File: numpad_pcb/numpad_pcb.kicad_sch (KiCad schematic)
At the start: 35 parts, among them J1 numpad, J10 Conn_01x02, J11 Conn_01x02, J12 Conn_01x02, J13 Conn_01x02, J14 Conn_01x02, J15 Conn_01x02, J17 Conn_01x02, J2 Conn_01x02, J3 Conn_01x02, J4 Conn_01x02, J6 Conn_01x02, J7 Conn_01x02, J8 Conn_01x02, J9 Conn_01x02, U1 ProMicro

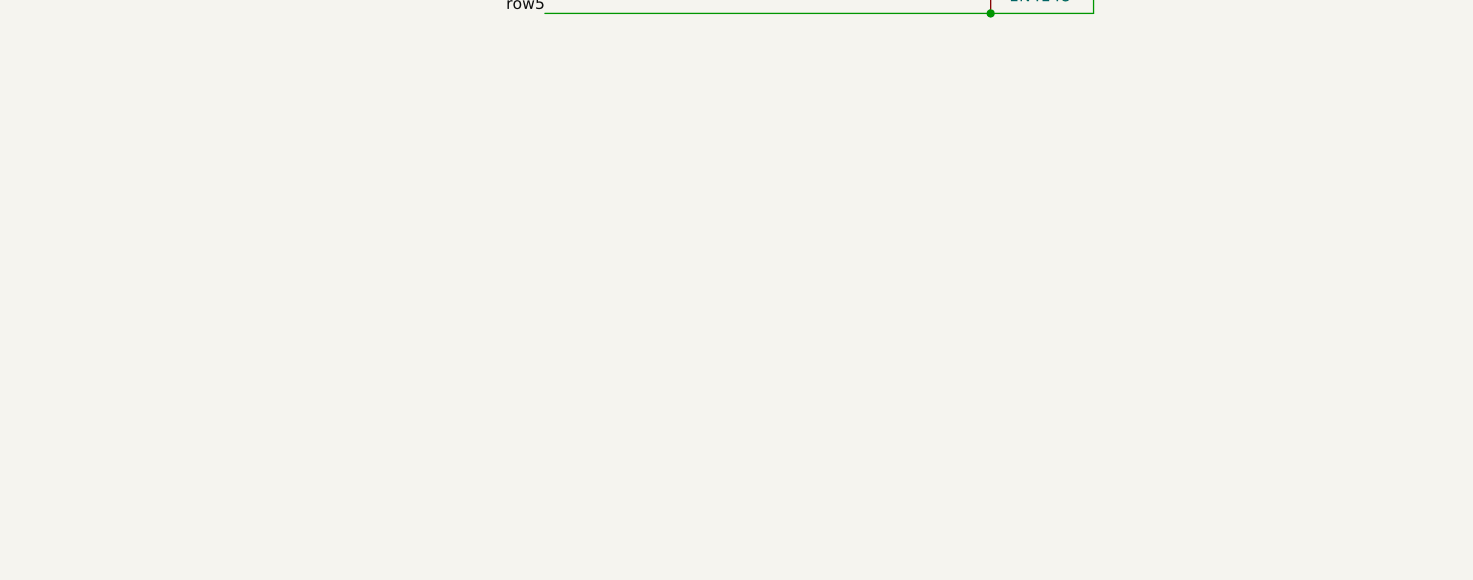
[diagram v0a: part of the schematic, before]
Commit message: tweaked silk, added todo for upgraded layout, added config
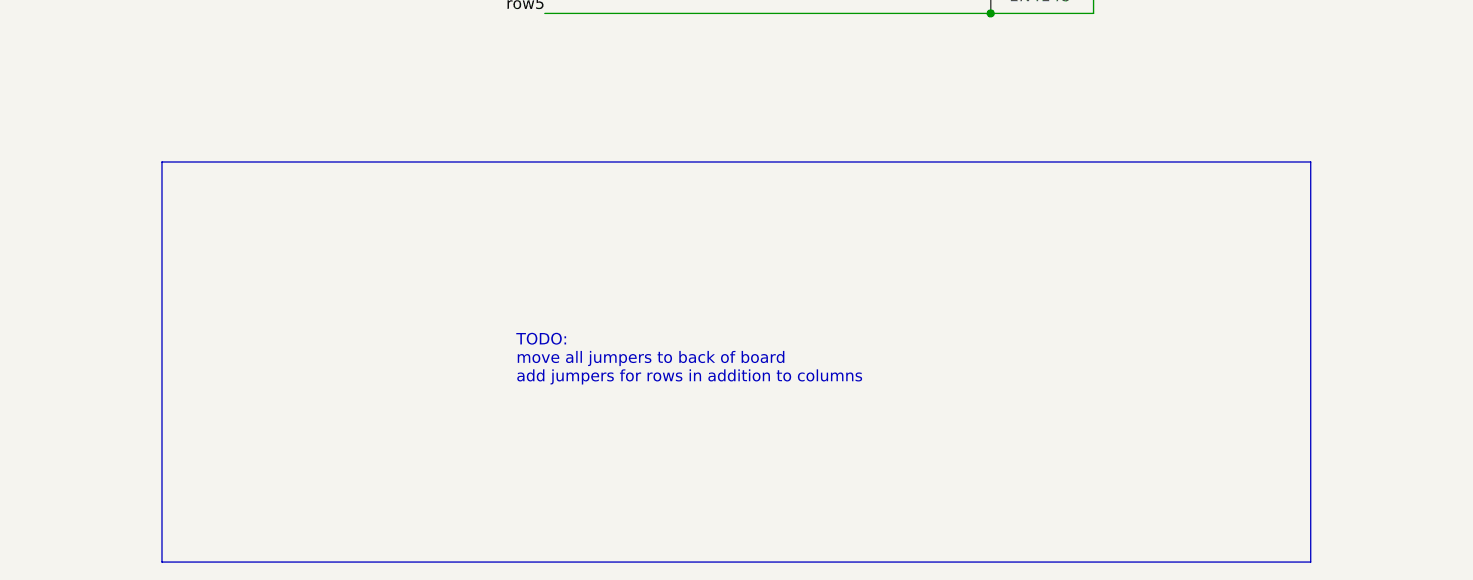
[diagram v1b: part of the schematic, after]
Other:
- note added: "TODO: move all jumpers to back of board add jumpers for rows in addition to columns"
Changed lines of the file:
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@@
+    (stroke (width 0) (type default) (color 0 0 0 0))
+  )
+  (polyline (pts (xy 34.925 147.32) (xy 34.925 191.77))
     (stroke (width 0) (type default) (color 0 0 0 0))
   )
@@
     (stroke (width 0) (type default) (color 0 0 0 0))
   )
+  (polyline (pts (xy 34.925 147.32) (xy 162.56 147.32))
+    (stroke (width 0) (type default) (color 0 0 0 0))
+  )
   (wire (pts (xy 212.09 105.41) (xy 236.22 105.41))
     (stroke (width 0) (type default) (color 0 0 0 0))
@@
     (stroke (width 0) (type default) (color 0 0 0 0))
   )
+  (polyline (pts (xy 162.56 147.32) (xy 162.56 191.77))
+    (stroke (width 0) (type default) (color 0 0 0 0))
+  )
   (wire (pts (xy 212.09 44.45) (xy 212.09 48.895))
     (stroke (width 0) (type default) (color 0 0 0 0))
@@
     (stroke (width 0) (type default) (color 0 0 0 0))
   )
+  (polyline (pts (xy 162.56 191.77) (xy 34.925 191.77))
+    (stroke (width 0) (type default) (color 0 0 0 0))
+  )
   (wire (pts (xy 96.52 44.45) (xy 96.52 48.895))
     (stroke (width 0) (type default) (color 0 0 0 0))
@@
     (stroke (width 0) (type default) (color 0 0 0 0))
   )
+  (text "TODO:\nmove all jumpers to back of board\nadd jumpers for rows in addition to columns"
+    (at 74.295 172.085 0)
+    (effects (font (size 1.27 1.27)) (justify left bottom))
+  )
   (label "row2" (at 76.2 71.12 180)

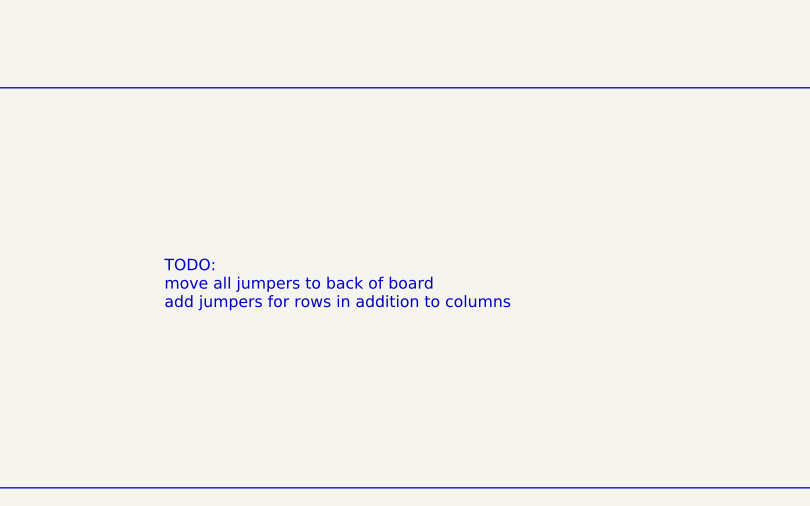
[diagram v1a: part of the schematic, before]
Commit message: tweaked schematic
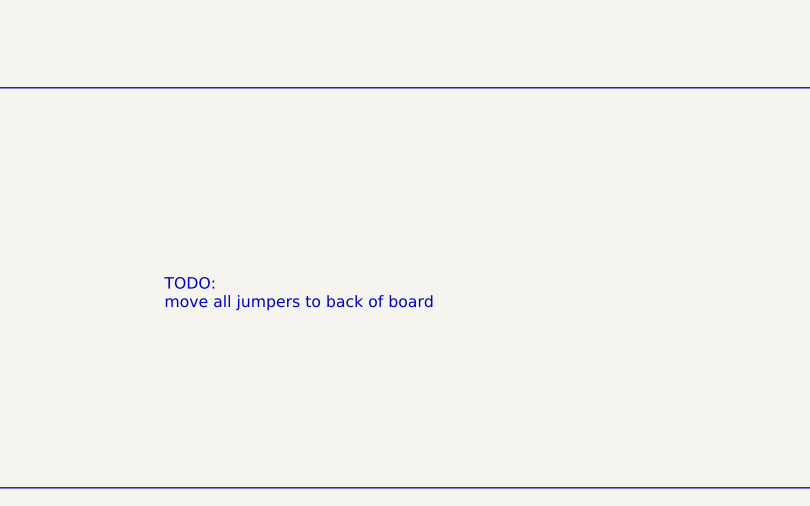
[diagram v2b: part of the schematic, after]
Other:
- note added: "TODO: move all jumpers to back of board"
- note removed: "TODO: move all jumpers to back of board add jumpers for rows in addition to columns"
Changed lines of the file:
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@@
     (stroke (width 0) (type default) (color 0 0 0 0))
   )
-  (text "TODO:\nmove all jumpers to back of board\nadd jumpers for rows in addition to columns"
-    (at 74.295 172.085 0)
+  (text "TODO:\nmove all jumpers to back of board" (at 74.295 172.085 0)
     (effects (font (size 1.27 1.27)) (justify left bottom))
   )

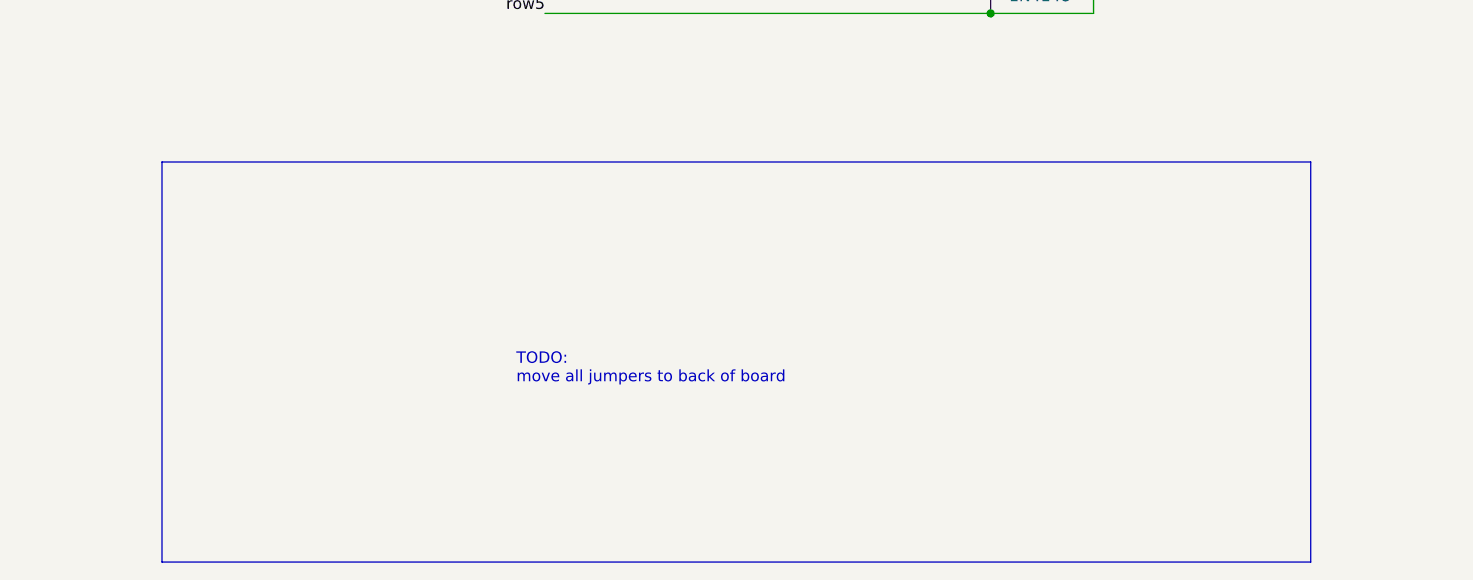
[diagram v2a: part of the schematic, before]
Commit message: moved jumpers to the back
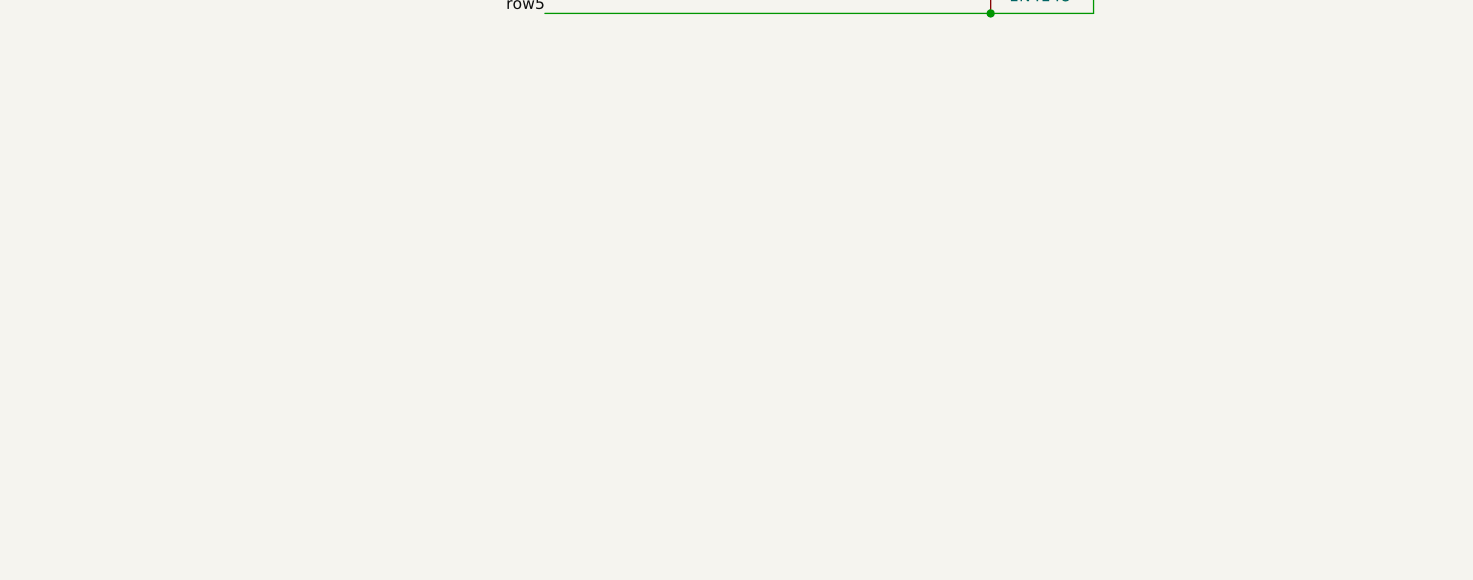
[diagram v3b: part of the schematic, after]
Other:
- note removed: "TODO: move all jumpers to back of board"
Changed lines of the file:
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@@
-    (stroke (width 0) (type default) (color 0 0 0 0))
-  )
-  (polyline (pts (xy 34.925 147.32) (xy 34.925 191.77))
     (stroke (width 0) (type default) (color 0 0 0 0))
   )
@@
     (stroke (width 0) (type default) (color 0 0 0 0))
   )
-  (polyline (pts (xy 34.925 147.32) (xy 162.56 147.32))
-    (stroke (width 0) (type default) (color 0 0 0 0))
-  )
   (wire (pts (xy 212.09 105.41) (xy 236.22 105.41))
     (stroke (width 0) (type default) (color 0 0 0 0))
@@
     (stroke (width 0) (type default) (color 0 0 0 0))
   )
-  (polyline (pts (xy 162.56 147.32) (xy 162.56 191.77))
-    (stroke (width 0) (type default) (color 0 0 0 0))
-  )
   (wire (pts (xy 212.09 44.45) (xy 212.09 48.895))
     (stroke (width 0) (type default) (color 0 0 0 0))
@@
     (stroke (width 0) (type default) (color 0 0 0 0))
   )
-  (polyline (pts (xy 162.56 191.77) (xy 34.925 191.77))
-    (stroke (width 0) (type default) (color 0 0 0 0))
-  )
   (wire (pts (xy 96.52 44.45) (xy 96.52 48.895))
     (stroke (width 0) (type default) (color 0 0 0 0))
@@
     (stroke (width 0) (type default) (color 0 0 0 0))
   )
-  (text "TODO:\nmove all jumpers to back of board" (at 74.295 172.085 0)
-    (effects (font (size 1.27 1.27)) (justify left bottom))
-  )
   (label "row2" (at 76.2 71.12 180)
